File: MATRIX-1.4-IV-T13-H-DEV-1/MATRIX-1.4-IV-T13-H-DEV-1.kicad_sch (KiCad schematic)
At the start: 222 parts, among them Q401 2N5551, Q402 2N5551, Q403 MJE340, Q404 MJE350, Q405 MJE350, Q406 MJE350, Q407 MJE340, Q408 MJE350, Q409 MJE340, Q410 MJE15032, Q411 MJE15033, Q412 2SC5200, Q413 2SA1943, Q4141 2SC5200, Q41410 2SC5200, Q4142 2SC5200, Q4143 2SC5200, Q4144 2SC5200, Q4145 2SC5200, Q4146 2SC5200, Q4147 2SC5200, Q4148 2SC5200, Q4149 2SC5200, Q4151 2SA1943, Q41510 2SA1943, Q4152 2SA1943, Q4153 2SA1943, Q4154 2SA1943, Q4155 2SA1943, Q4156 2SA1943, Q4157 2SA1943, Q4158 2SA1943, Q4159 2SA1943, Q501 2N5401, Q502 2N5551, Q503 2N5401, Q504 2N5551, Q505 2N5551, Q506 2N5401, Q507 2N5551, Q508 2N5551, Q509 TIP41C, Q601 2N5551, Q602 2N5401, Q603 2N5401, Q604 2N5401, Q605 2N5401, Q606 2N5551, Q607 BF423, Q701 2N5401, Q702 2N5551, Q703 2N5551, Q704 2N5551, Q705 2N5551, Q706 2N5401, Q707 BF422

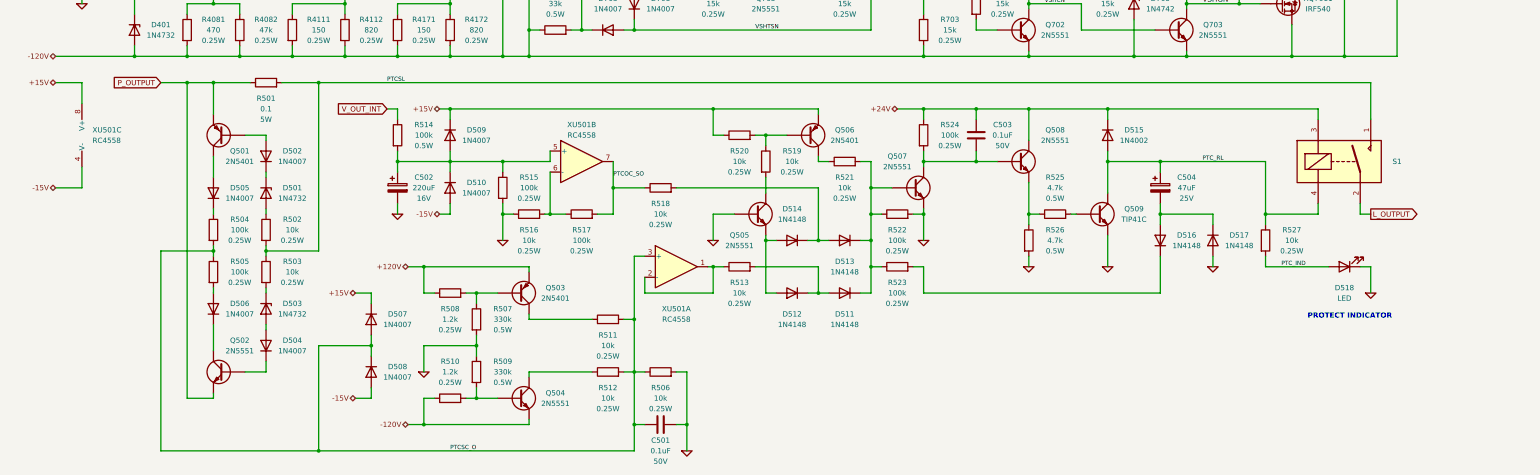
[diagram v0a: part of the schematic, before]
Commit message: Routine Update Sat Jun 18 06:40:31 PM WIB 2022
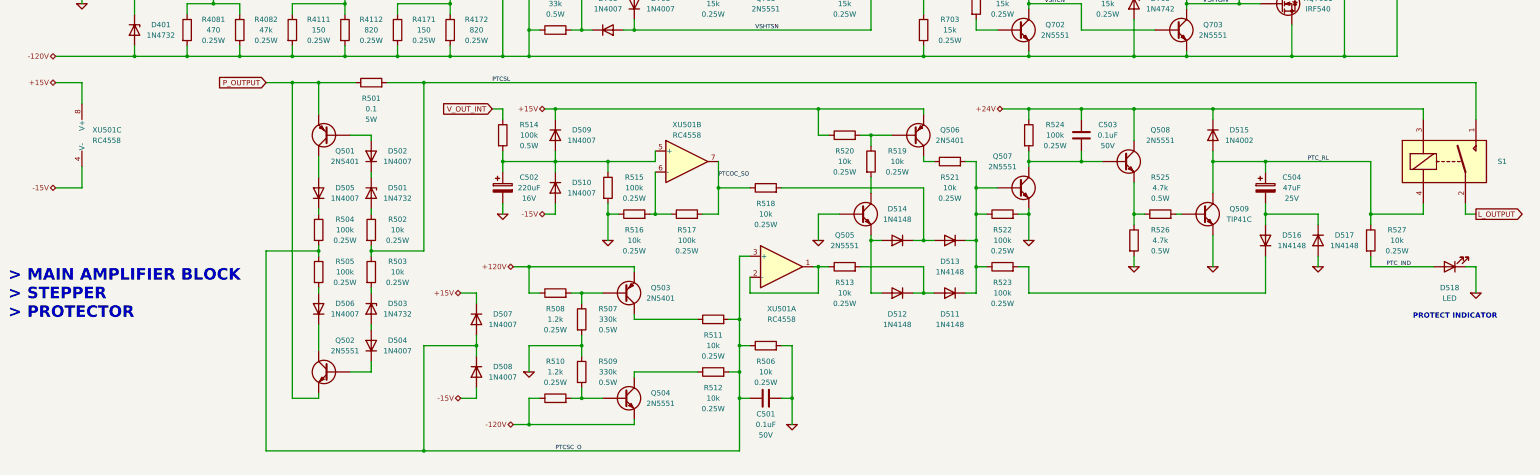
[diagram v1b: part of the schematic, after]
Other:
- note added: "> MAIN AMPLIFIER BLOCK > STEPPER > PROTECTOR"
- moved on the sheet: C501, C502, C503, C504, D501, D502, D503, D504, D505, D506, D507, D508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
